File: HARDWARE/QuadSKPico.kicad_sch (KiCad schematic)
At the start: 134 parts, among them J1 BOOT, J2 ADDR, J3 AVR-JTAG-10, J4 Conn_02x03_Odd_Even, J5 MONO, J6 HEADPHONE OUT, J7 EVO64 SID2 Pin27, P1 USB_C_Plug_USB2.0, U1 AP7365-33EG-13, U10 PCM5122PW, U11 PCM5122PW, U12 PCM5122PW, U13 TS3USB221EDRC, U14 MAX9723, U15 TXS0108EPW, U16 TXS0108EPW, U17 W25Q32RVXHJQ, U18 W25Q32RVXHJQ, U19 W25Q32RVXHJQ, U2 ATF1502ASL-xAx44, U20 W25Q32RVXHJQ, U3 RP2040, U4 RP2040, U5 RP2040, U6 RP2040, U7 OPA2134, U8 TS3USB221EDRC, U9 PCM5122PW, X1 DSC1001BI2-012.0000T

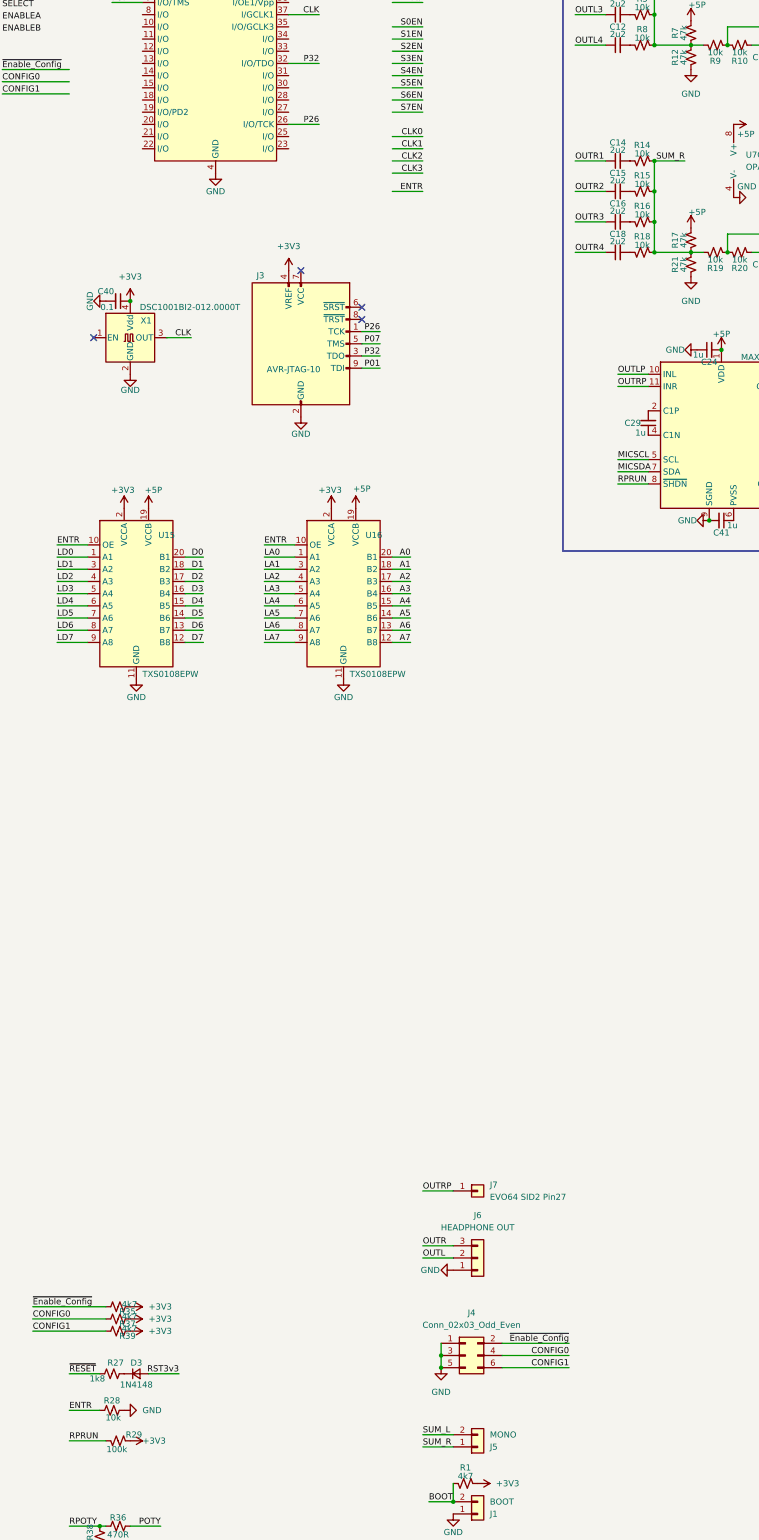
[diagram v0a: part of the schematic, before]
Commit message: Add files via upload
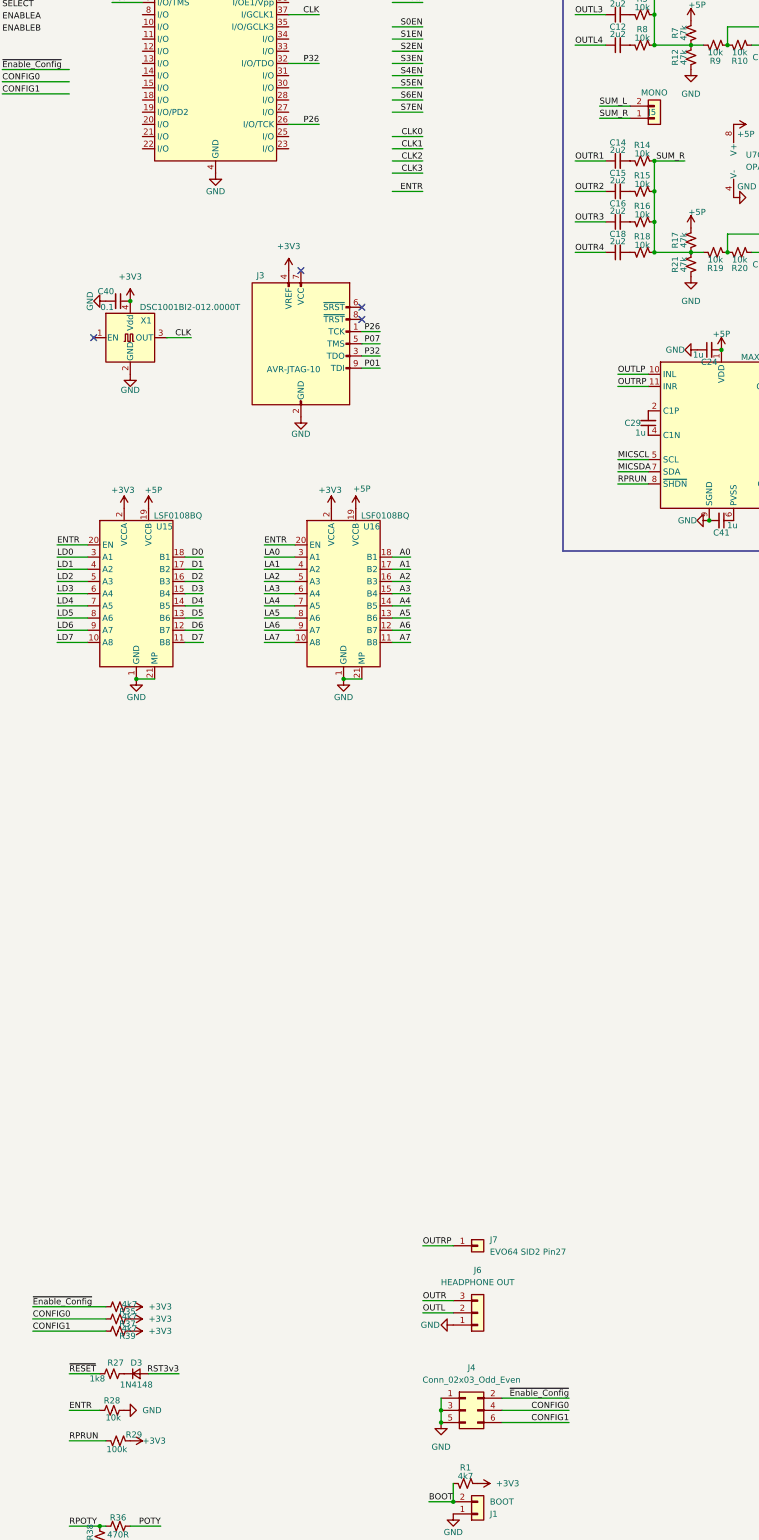
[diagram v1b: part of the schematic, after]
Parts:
- removed U15, U16: TXS0108EPW, Package_SO:TSSOP-20_4.4x6.5mm_P0.65mm, symbol Logic_LevelTranslator:TXS0108EPW
- added U15, U16: LSF0108BQ, Package_DFN_QFN:DHVQFN-20-1EP_2.5x4.5mm_P0.5mm_EP1x3mm, symbol CPU2:LSF0108BQ
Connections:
- net +3V3: now also U15.2 (VCCA), U16.2 (VCCA)
- net +5P: now also U15.19 (VCCB), U16.19 (VCCB)
- net A0: now also U16.18 (B1)
- net A1: now also U16.17 (B2)
- net A2: now also U16.16 (B3)
- net A3: now also U16.15 (B4)
- net A4: now also U16.14 (B5)
- net A5: now also U16.13 (B6)
- net A6: now also U16.12 (B7)
- net A7: now also U16.11 (B8)
- net D0: now also U15.18 (B1)
- net D1: now also U15.17 (B2)
- net D2: now also U15.16 (B3)
- net D3: now also U15.15 (B4)
- net D4: now also U15.14 (B5)
- net D5: now also U15.13 (B6)
- net D6: now also U15.12 (B7)
- net D7: now also U15.11 (B8)
- net ENTR: now also U15.20 (EN), U16.20 (EN)
- net EP: now also U15.1 (GND), U15.21 (MP), U16.1 (GND), U16.21 (MP)
- net LA0: now also U16.3 (A1)
- net LA1: now also U16.4 (A2)
- net LA2: now also U16.5 (A3)
- net LA3: now also U16.6 (A4)
- net LA4: now also U16.7 (A5)
- net LA5: now also U16.8 (A6)
- net LA6: now also U16.9 (A7)
- net LA7: now also U16.10 (A8)
- net LD0: now also U15.3 (A1)
- net LD1: now also U15.4 (A2)
- net LD2: now also U15.5 (A3)
- net LD3: now also U15.6 (A4)
- net LD4: now also U15.7 (A5)
- net LD5: now also U15.8 (A6)
- net LD6: now also U15.9 (A7)
- net LD7: now also U15.10 (A8)
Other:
- moved on the sheet: J4, J5, J6, J7
